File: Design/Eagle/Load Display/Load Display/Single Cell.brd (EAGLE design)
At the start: 68.2 x 83.8 mm, 12 parts

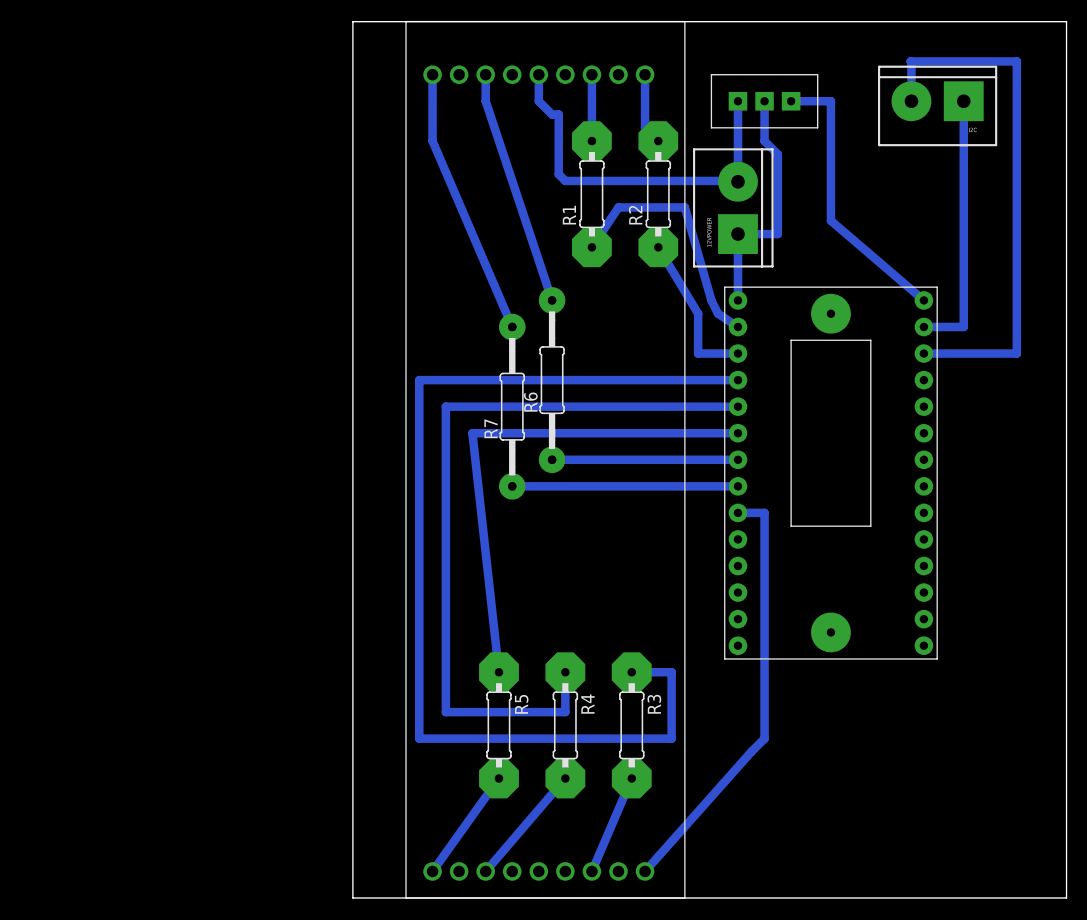
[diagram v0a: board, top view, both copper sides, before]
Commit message: Merge remote-tracking branch 'remotes/origin/Panic_Mode_Ben' into HEAD
Conflicts:
	Python/Master.py
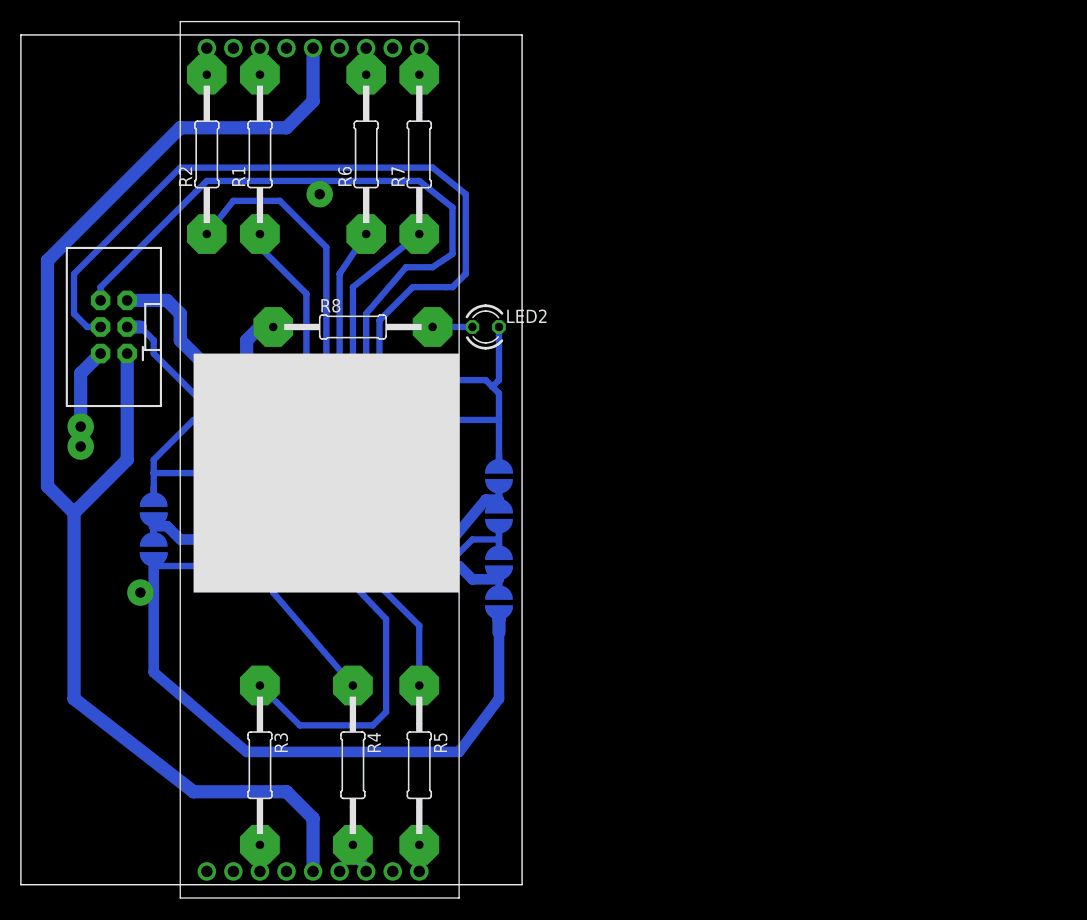
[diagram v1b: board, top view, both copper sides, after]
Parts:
- removed 12VPOWER, I2C: M025MM, Ben-SF-Con:SCREWTERMINAL-5MM-2
- added JP2: (no value), Ben-SF-Con:2X3-SHROUDED
- added LED2: TLLR4400, led:LED3MM
- added R8: 1000, Ben-rcl:0207/15
- added U$2: (no value), Parts:DRIVER_BOARD_ADAFRUIT
- added U$4, U$5, U$6, U$7: SOLDER_JUMPER, Parts:SOLDER_JUMPER
- added U$8: (no value), Parts:DRIVER_BOARD
- DIS1: device Parts:4INTESTER -> Parts:7SEGMENT_BACKWARDS
- R1, R2, R3, R4, R5: device Ben-rcl:0207/10 -> Ben-rcl:0207/15
- U$1: value 5VREG -> SOLDER_JUMPER; device Parts:LM78XX -> Parts:SOLDER_JUMPER
- U$3: value HT16K33BRD -> SOLDER_JUMPER; device Parts:HT16K33BRKOUT -> Parts:SOLDER_JUMPER
- moved U$1 53.4 mm to (45.7, 26.7), flipped to the bottom, turned to 180 degrees
- moved R2 43.3 mm to (17.8, 69.9)
- moved R3 35.8 mm to (22.9, 11.4)
- moved R1 32.0 mm to (22.9, 69.9)
- moved R6 28.0 mm to (33.0, 69.9)
- moved R7 25.7 mm to (38.1, 69.9)
- moved U$3 24.1 mm to (45.7, 30.5), flipped to the bottom, turned to 180 degrees
- moved DIS1 21.6 mm to (17.8, 1.27)
- moved R4 20.7 mm to (31.7, 11.4)
- moved R5 8.52 mm to (38.1, 11.4)
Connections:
- removed net N$19: U$1.P$3, U$3.VDD
- removed net N$20: 12VPOWER.2, DIS1.8, U$1.P$1
- new net GND: JP2.2, JP2.6, LED2.K, U$1.P$1, U$2.G, U$2.GND, U$4.P$1, U$6.P$1, U$8.G, U$8.GND
- new net N$29: U$1.P$2, U$2.A0, U$3.P$1, U$8.A0
- new net SDA: JP2.3, U$2.SDA, U$8.SDA
- new net SSCL: JP2.4, U$2.SCL, U$8.SCL
- new net VCC12: DIS1.3, DIS1.8, JP2.1
- new net VCC5: JP2.5, R8.1, U$2.VCC, U$3.P$2, U$5.P$2, U$7.P$2, U$8.VCC
- net N$10: now also U$2.DRAIN2, U$8.DRAIN2; no longer U$3.C2
- net N$11: now also U$2.DRAIN3, U$8.DRAIN3; no longer U$3.C3
- net N$12: now also U$2.DRAIN4, U$8.DRAIN4; no longer U$3.C4
- net N$13: now also U$2.DRAIN5, U$8.DRAIN5; no longer U$3.C5
- net N$14: now also U$2.DRAIN6, U$8.DRAIN6; no longer U$3.C6
- net N$15: now also U$2.A1, U$4.P$2, U$5.P$1, U$8.A1; no longer I2C.1, U$3.SDA
- net N$16: now also U$2.A2, U$6.P$2, U$7.P$1, U$8.A2; no longer I2C.2, U$3.SCL
- net N$17: now also U$2.DRAIN7, U$8.DRAIN7; no longer 12VPOWER.1, U$1.P$2, U$3.GND
- net N$18: now also LED2.A, R8.2; no longer DIS1.5, U$3.C7
- net N$8: now also U$2.DRAIN0, U$8.DRAIN0; no longer U$3.C0
- net N$9: now also U$2.DRAIN1, U$8.DRAIN1; no longer U$3.C1
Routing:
- net GND: track 0.00 -> 172.5 mm
- net VCC12: track 0.00 -> 129.1 mm
- net VCC5: track 0.00 -> 93.9 mm
- net SSCL: track 0.00 -> 79.7 mm
- net N$10: track 99.1 -> 44.4 mm
- net N$11: track 72.4 -> 23.7 mm
- net N$16: track 50.8 -> 9.42 mm
- net N$18: track 41.2 -> 3.81 mm
- net N$20: track 35.8 -> 0.00 mm, vias 0 -> 1
- net N$9: track 15.0 -> 43.8 mm
- net N$19: track 26.9 -> 0.00 mm, vias 0 -> 1
- net N$7: track 25.7 -> 2.54 mm
- net N$12: track 48.4 -> 25.9 mm
- net N$17: track 23.4 -> 2.54 mm
- net N$6: track 22.6 -> 2.54 mm
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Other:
- board size 68.2 x 83.8 mm -> 47.9 x 81.3 mm
